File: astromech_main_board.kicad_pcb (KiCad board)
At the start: 2 copper layers, 76.2 x 88.9 mm, 75 parts, among them IC1 MAX11645EUA+, J1 Conn_01x03, J10 61201621621, J11 Conn_01x06, J15 Conn_01x04, J18 Screw_Terminal_01x10, J19 Conn_01x04, J2 Conn_02x03_Odd_Even, J20 Conn_01x04, J21 Conn_01x04, J3 Conn_01x03, J4 IO_XPAND, J7 Conn_01x03, J8 Conn_01x03, J9 Conn_01x06, Q1 2N7002, U10 LS7366R, U11 LS7366R, U3 NCP1117-3.3_SOT223, U4 NCP1117-5.0_TO252, U5 SC16IS752IPW_128, U6 PCF8575PWR, U7 TCA9517ADGK, U8 74HC14, U9 LS7366R, Y1 8MHz, Y2 Crystal

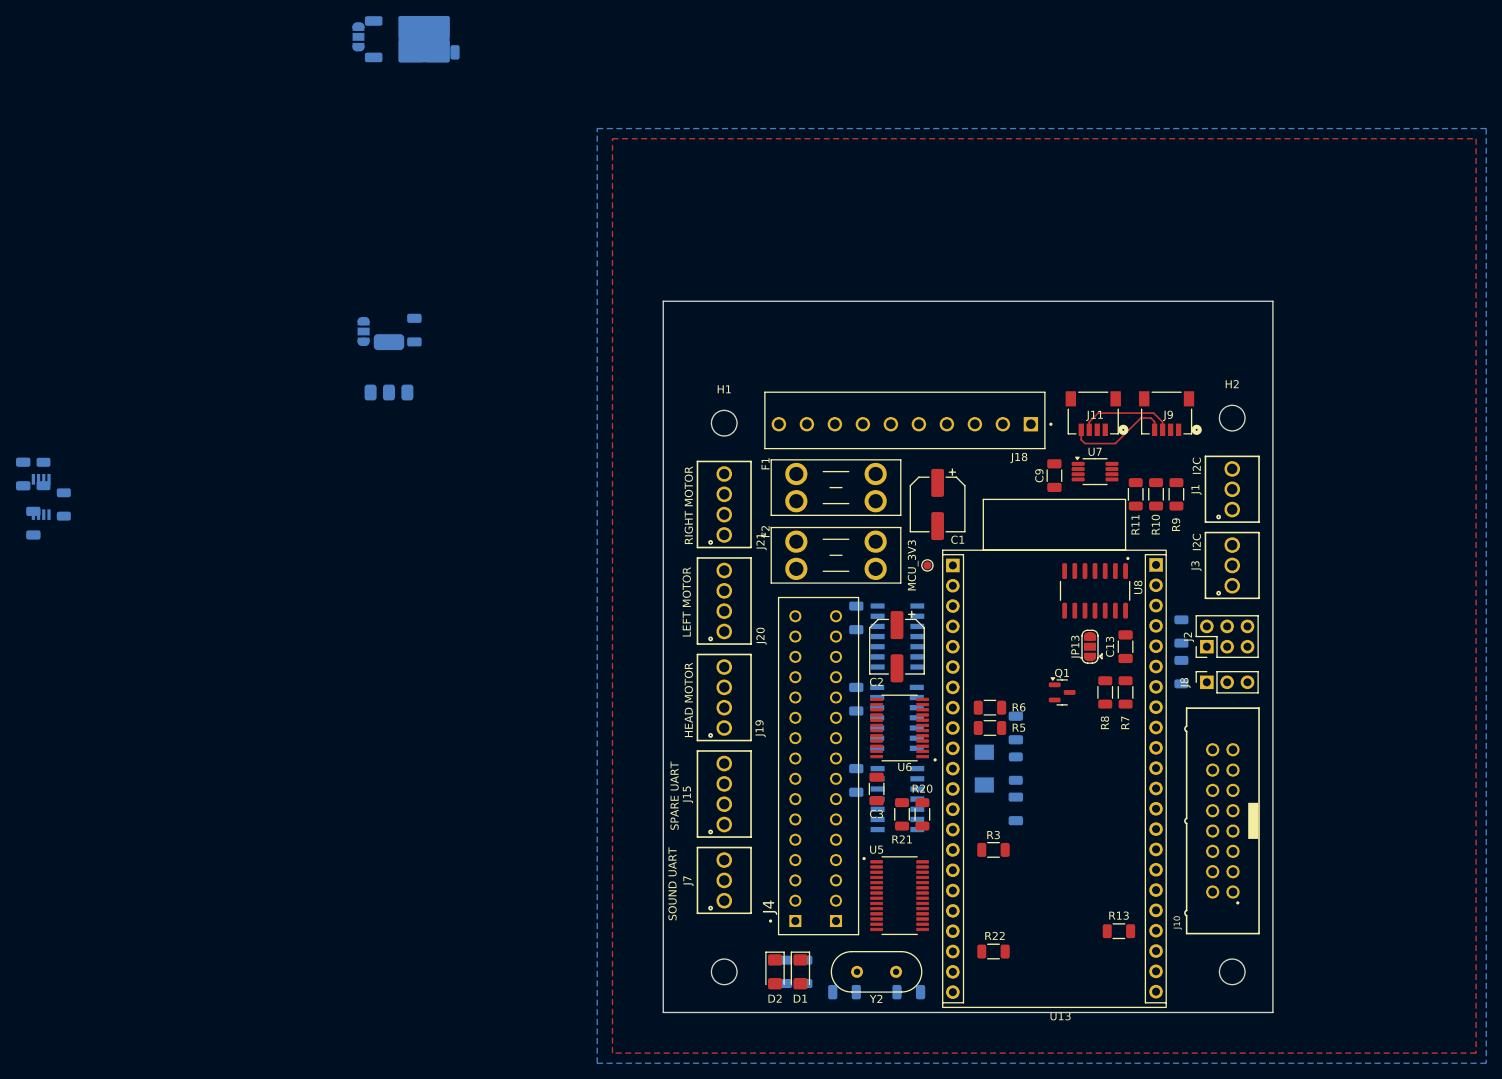
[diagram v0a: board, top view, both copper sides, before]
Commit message: new layout done
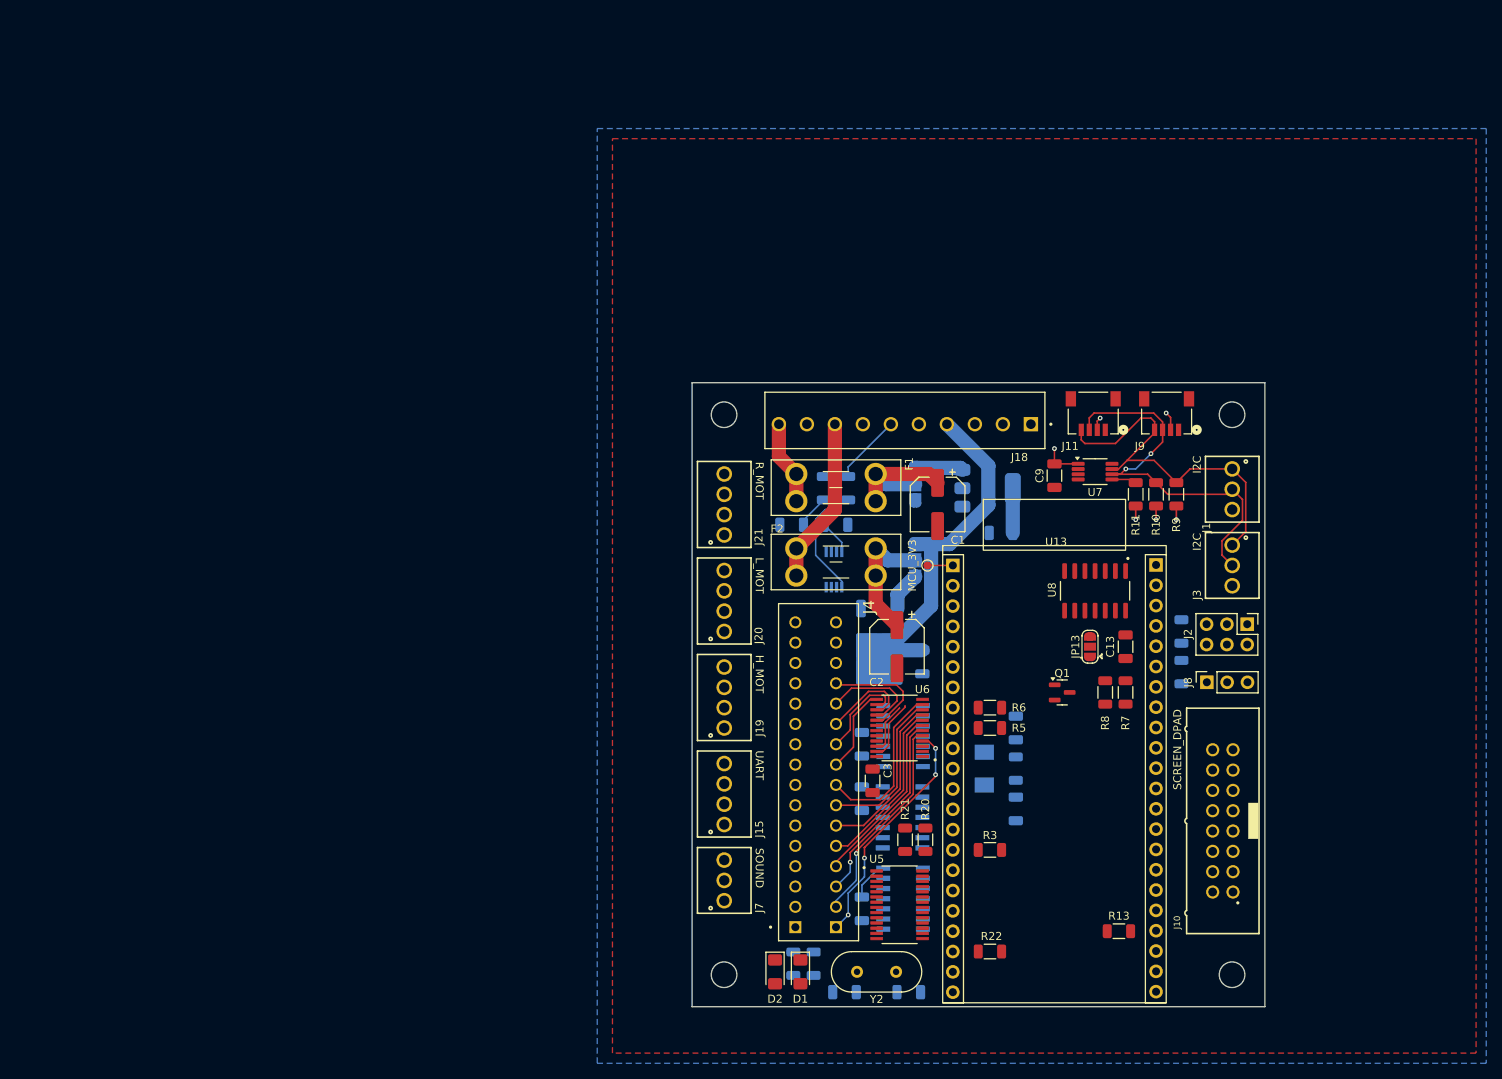
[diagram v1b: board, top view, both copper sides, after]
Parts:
- moved C16 100.3 mm to (174.0, 86.4), turned to 180 degrees
- moved IC1 99.5 mm to (173.7, 91.9)
- moved R1 98.1 mm to (175.5, 81.8)
- moved R2 97.6 mm to (172.5, 81.8)
- moved C15 96.9 mm to (184.8, 103.5), turned to -90 degrees
- moved C17 96.3 mm to (168.5, 86.4), turned to 0 degrees
- moved U4 95.9 mm to (179.4, 101.9), turned to -90 degrees
- moved JP8 95.5 mm to (183.9, 90.8), turned to -90 degrees
- moved C14 77.6 mm to (194.6, 87.4), turned to 180 degrees
- moved U3 76.3 mm to (192.9, 81.8), turned to 0 degrees
- moved JP7 71.6 mm to (183.9, 81.3), turned to 90 degrees
- moved C10 16.1 mm to (177.2, 134.4)
- moved C12 15.8 mm to (177.2, 113.8)
- moved U10 12.5 mm to (182.3, 122.9)
- moved C11 12.5 mm to (177.2, 120.6)
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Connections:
- U13 pad 8: /I2C_3V3_SDA -> /I2C_3V3_SCL
- U13 pad 9: /I2C_3V3_SCL -> /I2C_3V3_SDA
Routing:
- net 5V: track 0.00 -> 42.3 mm
- net /SDA_BUFD: track 12.1 -> 49.9 mm, vias 0 -> 2
- net /SCL_BUFD: track 13.1 -> 46.6 mm
- net Net-(D1-K): track 0.00 -> 29.6 mm, vias 0 -> 4
- net 3V3: track 0.00 -> 28.9 mm, vias 0 -> 6
- net Net-(D2-K): track 0.00 -> 26.3 mm, vias 0 -> 1
- net Net-(J4-Pin_3): track 0.00 -> 24.4 mm, vias 0 -> 1
- net Net-(J4-Pin_4): track 0.00 -> 22.5 mm
- net Net-(J4-Pin_5): track 0.00 -> 21.5 mm
- net Net-(IC1-AIN0): track 0.00 -> 20.9 mm
- net Net-(J18-Pin_8): track 0.00 -> 20.9 mm
- net Net-(J4-Pin_8): track 0.00 -> 20.8 mm
- net Net-(J4-Pin_6): track 0.00 -> 20.7 mm
- net Net-(J4-Pin_7): track 0.00 -> 20.0 mm
- net /3V3_IN: track 0.00 -> 17.1 mm
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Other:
- board size 76.2 x 88.9 mm -> 71.6 x 78 mm
- board text added: "GND"
